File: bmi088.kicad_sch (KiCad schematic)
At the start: 1 part, among them U1 BMI088

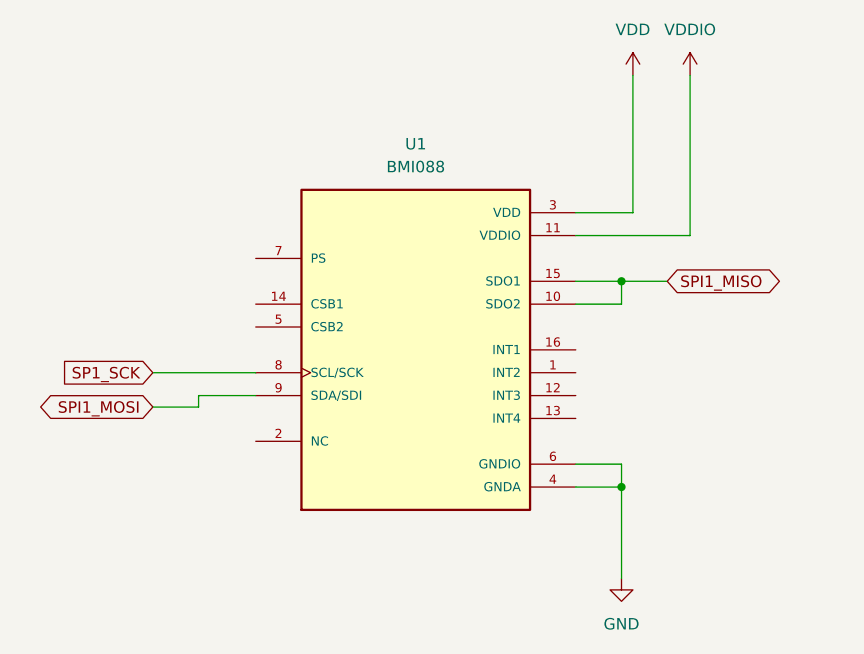
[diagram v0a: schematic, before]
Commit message: progress
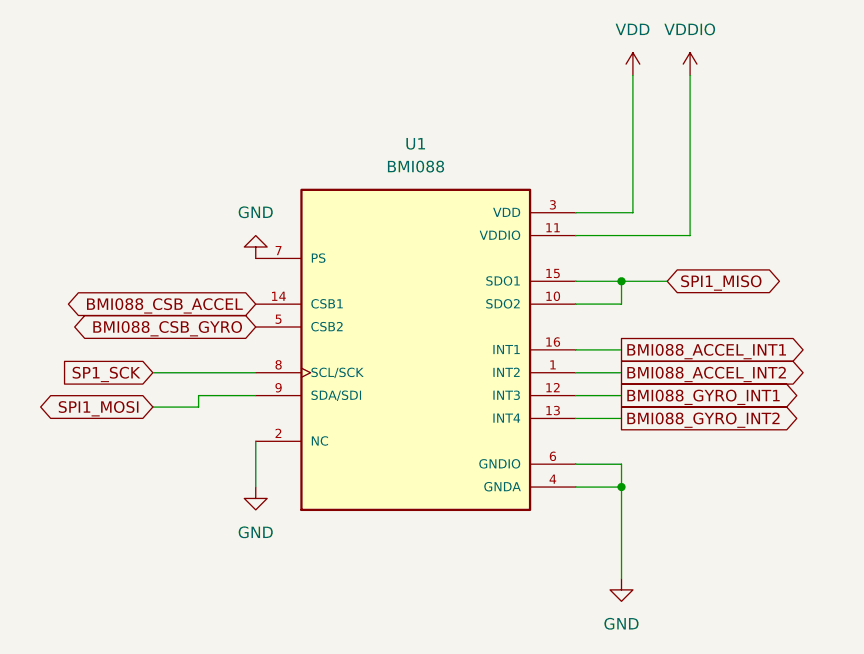
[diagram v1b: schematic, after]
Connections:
- net GND: now also U1.2 (NC), U1.7 (PS)
- net BMI088_ACCEL_INT2: now reaches U1.1 (INT2)
- net BMI088_GYRO_INT1: now reaches U1.12 (INT3)
- net BMI088_GYRO_INT2: now reaches U1.13 (INT4)
- net BMI088_CSB_ACCEL: now reaches U1.14 (CSB1)
- net BMI088_ACCEL_INT1: now reaches U1.16 (INT1)
- net BMI088_CSB_GYRO: now reaches U1.5 (CSB2)
